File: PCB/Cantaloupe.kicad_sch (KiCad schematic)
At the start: 118 parts, among them J1 RGB_Out, J2 SWD, J3 Trackpad, J4 OLED, J5 Extra, J6 USB_In, J7 Split_comm_link, Q1 AO3400A, Q2 AO3400A, SW1 MX, SW10 MX, SW11 MX, SW12 MX, SW13 MX, SW14 MX, SW15 MX, SW16 MX, SW17 MX, SW18 MX, SW19 MX, SW2 MX, SW20 MX, SW21 MX, SW22 MX, SW23 MX, SW24 MX, SW25 MX, SW26 MX, SW27 MX, SW28 MX, SW29 MX, SW3 MX, SW30 MX, SW31 Encoder, SW32 Reset, SW4 MX, SW5 MX, SW6 MX, SW7 MX, SW8 MX, SW9 MX, U1 STM32F411CCU6, U2 MB85RS64, U3 SRV05-4, U4 SRV05-4, U5 W25Q128JVS, U6 XC6220B331MR-G, Y1 8MHz

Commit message: Better routing
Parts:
- SW1, SW10, SW11, SW12, SW13, SW14, SW15, SW16, SW17, SW18, SW19, SW2, SW20, SW21, SW22, SW23, SW24, SW25, SW26, SW27, SW28, SW29, SW3, SW30, SW4, SW5, SW6, SW7, SW8, SW9: footprint Cantaloupe:MXOnly-1U-Hotswap-Dual -> Cantaloupe:MX_Choc-1U-Hotswap-Dual

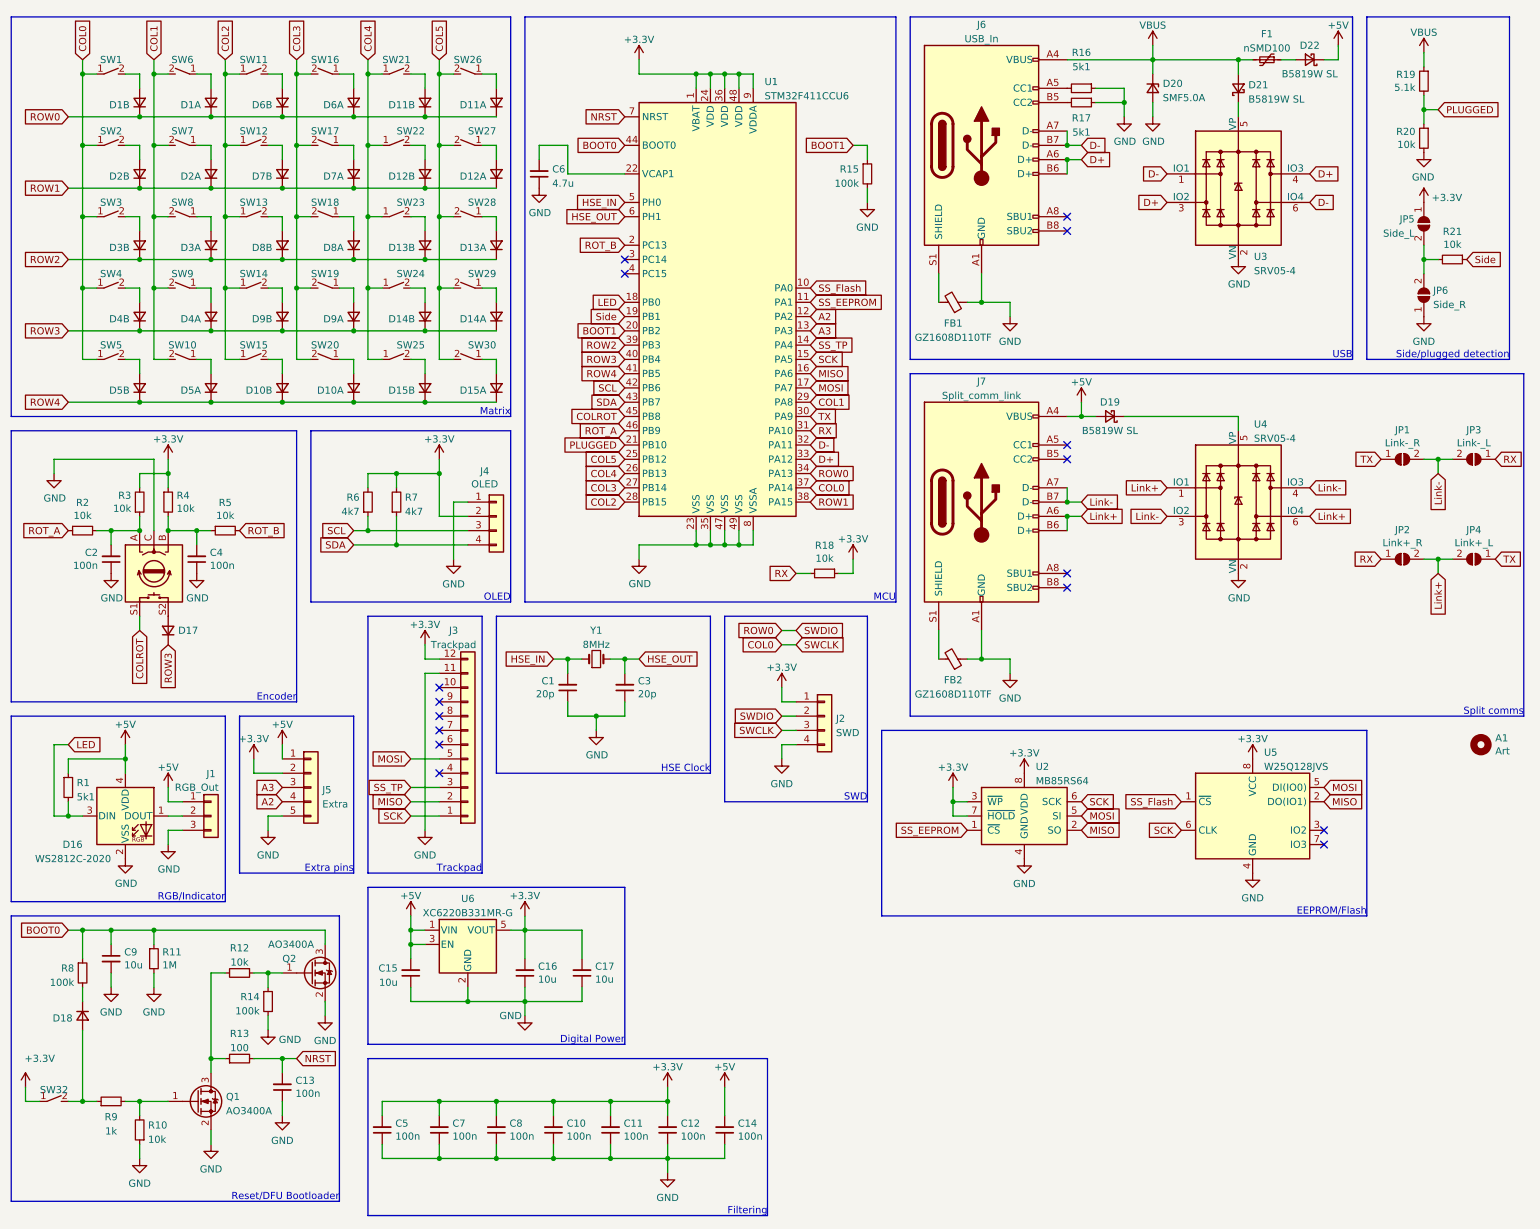
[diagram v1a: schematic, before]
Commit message: INCOMPLETE V3.0 Initial Update
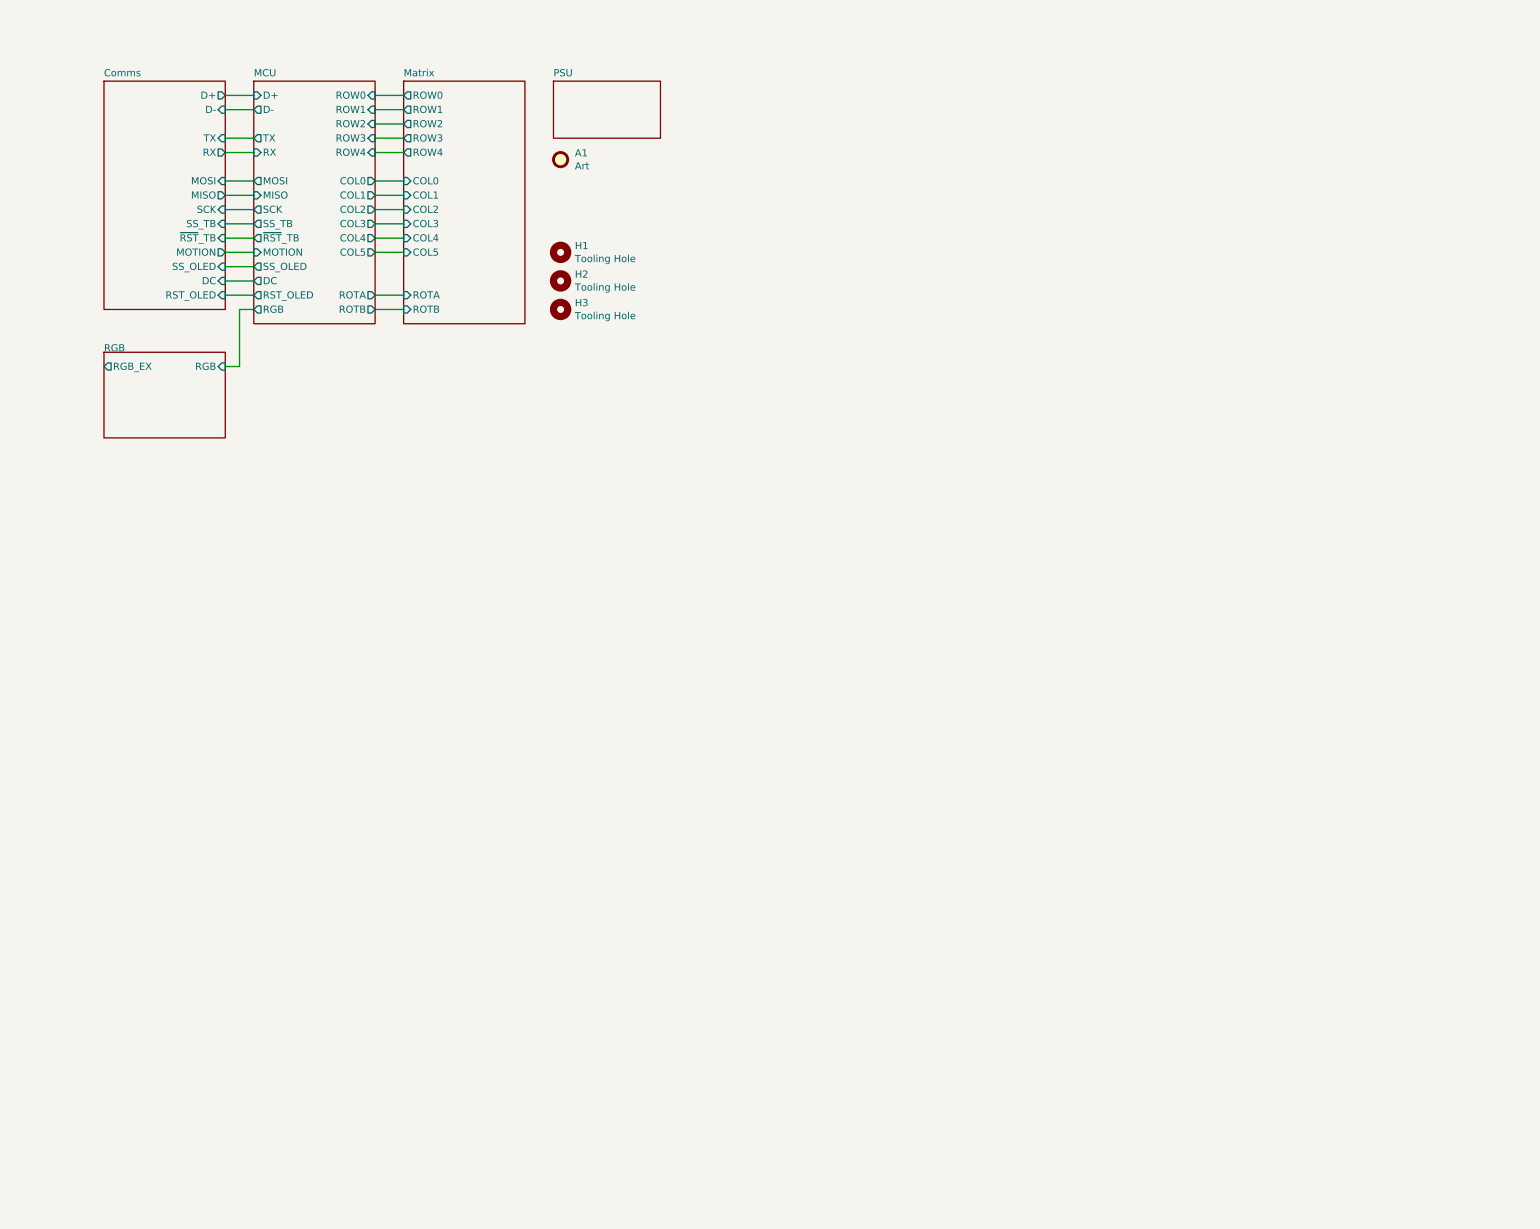
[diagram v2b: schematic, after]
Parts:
- removed C1, C3: 20p, Capacitor_SMD:C_0603_1608Metric, symbol Device:C_Small
- removed C10, C11, C12, C13, C14, C2, C4, C5, C7, C8: 100n, Capacitor_SMD:C_0603_1608Metric, symbol Device:C_Small
- removed C15, C16, C17, C9: 10u, Capacitor_SMD:C_0603_1608Metric, symbol Device:C_Small
- removed C6: 4.7u, Capacitor_SMD:C_0603_1608Metric, symbol Device:C_Small
- removed D1, D10, D11, D12, D13, D14, D15, D2, D3, D4, D5, D6, D7, D8, D9: D_Dual_CommonCathode_AAK_Split_Small, Package_TO_SOT_SMD:SOT-23, symbol Cantaloupe:D_Dual_CommonCathode_AAK_Split_Small
- removed D16: WS2812C-2020, Cantaloupe:LED_WS2812-2020_Flippable, symbol LED:SK6812MINI
- removed D17, D18: D, Cantaloupe:D_SOD-123, symbol Device:D_Small
- removed D19, D21, D22: B5819W SL, Cantaloupe:D_SOD-123, symbol Device:D_Schottky_Small
- removed D20: SMF5.0A, Cantaloupe:D_SOD-123, symbol Device:D_Zener_Small
- removed F1: nSMD100, Fuse:Fuse_1206_3216Metric, symbol Device:Polyfuse_Small
- removed FB1, FB2: GZ1608D110TF, Inductor_SMD:L_0603_1608Metric, symbol Djinn-rescue:Ferrite_Bead_Small-Device
- removed J1: RGB_Out, Cantaloupe:PinHeader_1x03_P2.54mm_Vertical_Silkless, symbol Connector_Generic:Conn_01x03
- removed J2: SWD, Cantaloupe:PinHeader_1x04_P2.54mm_Vertical_SIlkless, symbol Connector_Generic:Conn_01x04
- removed J3: Trackpad, Cantaloupe:Hirose_FH12-12S-0.5SH_1x12-1MP_P0.50mm_Horizontal_Flippable, symbol Connector_Generic:Conn_01x12
- removed J4: OLED, Cantaloupe:OLED_0.96_SSD1306_128x64_Flippable_Reversepads, symbol Connector_Generic:Conn_01x04
- removed J5: Extra, Cantaloupe:PinHeader_1x05_P2.54mm_Vertical_Silkless, symbol Connector_Generic:Conn_01x05
- removed J6: USB_In, Cantaloupe:HRO-TYPE-C-31-M-13x, symbol Cantaloupe:USB_C_Receptacle_USB2.0-Connector
- removed J7: Split_comm_link, Cantaloupe:HRO-TYPE-C-31-M-13x, symbol Cantaloupe:USB_C_Receptacle_USB2.0-Connector
- removed JP1: Link-_R, Jumper:SolderJumper-2_P1.3mm_Open_Pad1.0x1.5mm, symbol Jumper:SolderJumper_2_Open
- removed JP2: Link+_R, Jumper:SolderJumper-2_P1.3mm_Open_Pad1.0x1.5mm, symbol Jumper:SolderJumper_2_Open
- removed JP3: Link-_L, Jumper:SolderJumper-2_P1.3mm_Open_Pad1.0x1.5mm, symbol Jumper:SolderJumper_2_Open
- removed JP4: Link+_L, Jumper:SolderJumper-2_P1.3mm_Open_Pad1.0x1.5mm, symbol Jumper:SolderJumper_2_Open
- removed JP5: Side_L, Jumper:SolderJumper-2_P1.3mm_Open_Pad1.0x1.5mm, symbol Jumper:SolderJumper_2_Open
- removed JP6: Side_R, Jumper:SolderJumper-2_P1.3mm_Open_Pad1.0x1.5mm, symbol Jumper:SolderJumper_2_Open
- removed Q1, Q2: AO3400A, Package_TO_SOT_SMD:SOT-23, symbol Transistor_FET:AO3400A
- removed R1, R16, R17: 5k1, Resistor_SMD:R_0603_1608Metric, symbol Device:R_Small
- removed R10, R12, R18, R2, R20, R21, R3, R4, R5: 10k, Resistor_SMD:R_0603_1608Metric, symbol Device:R_Small
- removed R11: 1M, Resistor_SMD:R_0603_1608Metric, symbol Device:R_Small
- removed R13: 100, Resistor_SMD:R_0603_1608Metric, symbol Device:R_Small
- removed R14, R15, R8: 100k, Resistor_SMD:R_0603_1608Metric, symbol Device:R_Small
- removed R19: 5.1k, Resistor_SMD:R_0603_1608Metric, symbol Device:R_Small
- removed R6, R7: 4k7, Resistor_SMD:R_0603_1608Metric, symbol Device:R_Small
- removed R9: 1k, Resistor_SMD:R_0603_1608Metric, symbol Device:R_Small
- removed SW1, SW10, SW11, SW12, SW13, SW14, SW15, SW16, SW17, SW18, SW19, SW2, SW20, SW21, SW22, SW23, SW24, SW25, SW26, SW27, SW28, SW29, SW3, SW30, SW4, SW5, SW6, SW7, SW8, SW9: MX, Cantaloupe:MX_Choc-1U-Hotswap-Dual, symbol Cantaloupe:SW_SPST_Small
- removed SW31: Encoder, Cantaloupe:EC11_Flippable, symbol Device:Rotary_Encoder_Switch
- removed SW32: Reset, Cantaloupe:Switch_TS24ZJ_Flippable, symbol Cantaloupe:SW_SPST_Small
- removed U1: STM32F411CCU6, Package_DFN_QFN:QFN-48-1EP_7x7mm_P0.5mm_EP5.6x5.6mm, symbol MCU_ST_STM32F4:STM32F411CCUx
- removed U2: MB85RS64, Package_SO:SSOP-8_3.9x5.05mm_P1.27mm, symbol Memory_NVRAM:MB85RS64
- removed U3, U4: SRV05-4, Package_TO_SOT_SMD:SOT-23-6, symbol Power_Protection:SRV05-4
- removed U5: W25Q128JVS, Package_SO:SOIC-8_5.275x5.275mm_P1.27mm, symbol Memory_Flash:W25Q128JVS
- removed U6: XC6220B331MR-G, Package_TO_SOT_SMD:SOT-23-5, symbol Regulator_Linear:AP2112K-3.3
- removed Y1: 8MHz, Crystal:Crystal_SMD_5032-2Pin_5.0x3.2mm, symbol Device:Crystal_Small
- added H1, H2, H3: Tooling Hole, Cantaloupe:JLC Tooling Hole, symbol Mechanical:MountingHole
- A1: symbol Mechanical:MountingHole -> Mechanical:Fiducial; now in the parts list
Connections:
- no-connect marks 16 -> 0
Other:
- added sheet Comms (Comms.kicad_sch)
- added sheet MCU (MCU.kicad_sch)
- added sheet Matrix (Matrix.kicad_sch)
- added sheet PSU (PSU.kicad_sch)
- added sheet RGB (RGB.kicad_sch)
- note removed: "Digital Power"
- note removed: "EEPROM/Flash"
- note removed: "Encoder"
- note removed: "Extra pins"
- note removed: "Filtering"
- note removed: "HSE Clock"
- note removed: "MCU"
- note removed: "Matrix"
- note removed: "OLED"
- note removed: "RGB/Indicator"
- note removed: "Reset/DFU Bootloader"
- note removed: "SWD"
- note removed: "Side/plugged detection"
- note removed: "Split comms"
- note removed: "Trackpad"
- note removed: "USB"
